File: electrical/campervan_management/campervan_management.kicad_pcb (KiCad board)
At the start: 2 copper layers, 45 parts, among them J1 Duoetto Remote, J2 Input Flow Sensor, J3 Output Flow Sensor, J4 Battery Box, J5 Starter Battery, J6 Fuse and Switch Box, K1 G5Q-1, K2 G5Q-1, K3 G5Q-1, Q1 BC337, Q2 BC337, Q3 BC337, Q4 BC337, SW1 SW_Push, U1 RS485-TTL, U2 LM7805

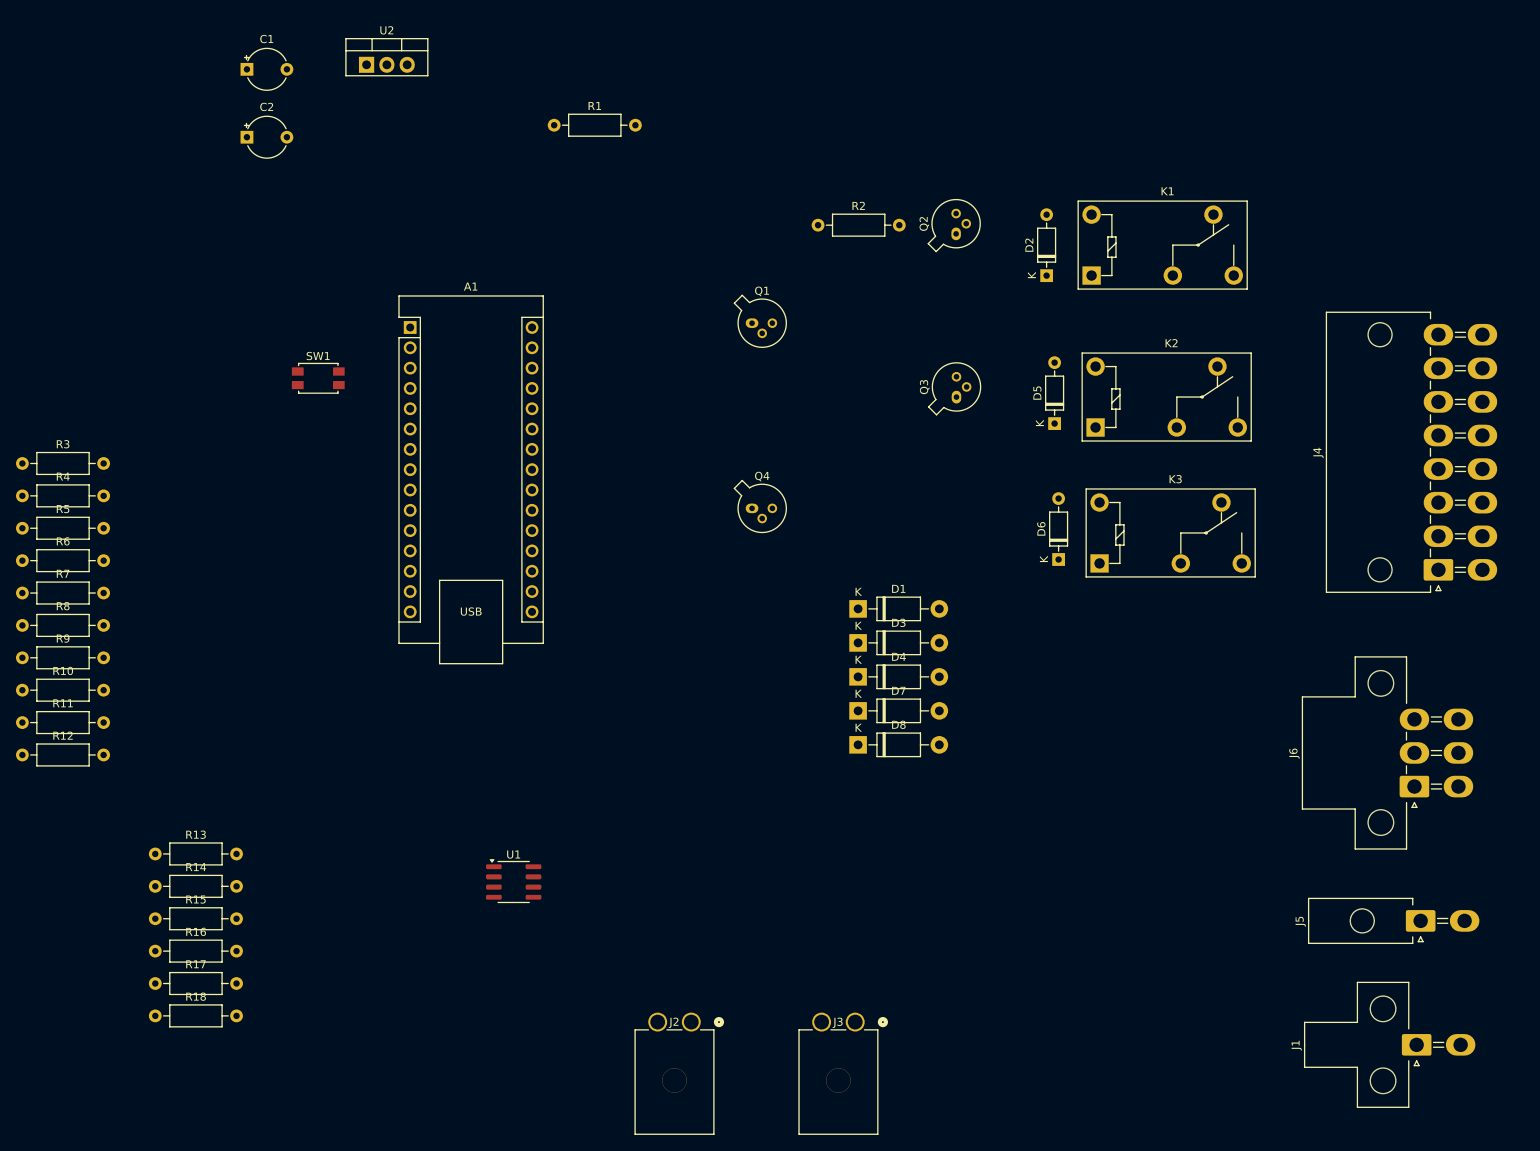
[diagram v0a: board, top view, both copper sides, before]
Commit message: First attempt at PCB design
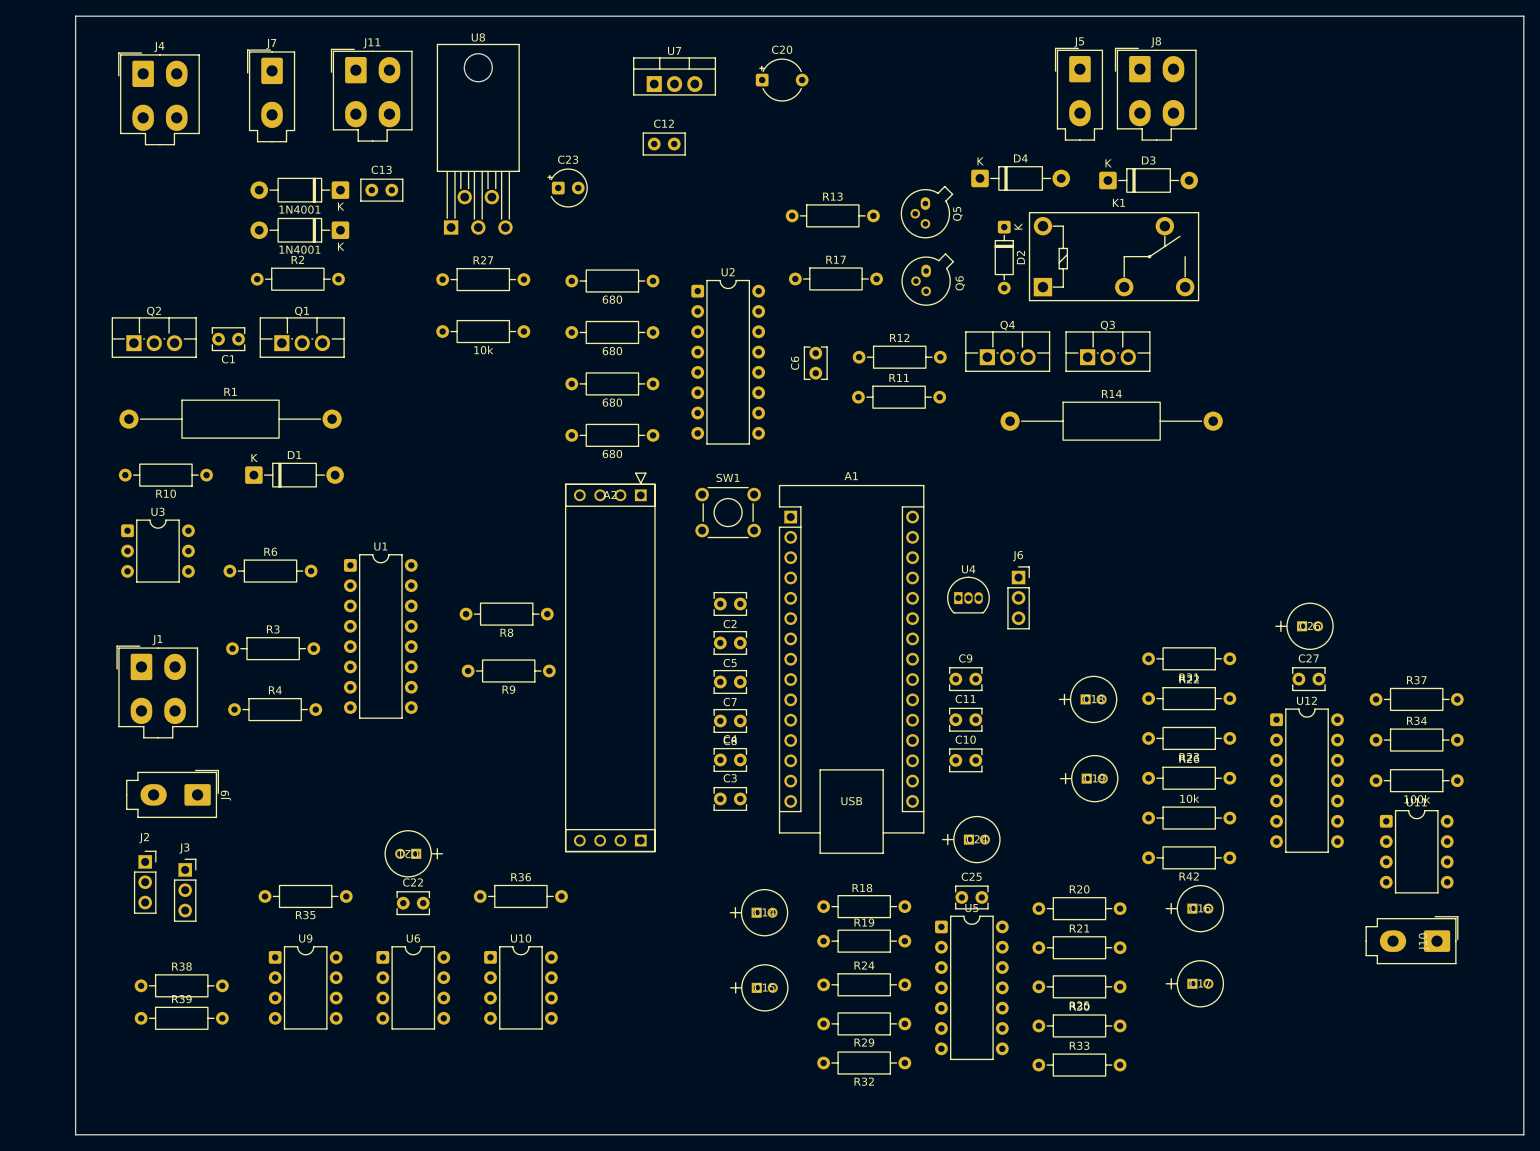
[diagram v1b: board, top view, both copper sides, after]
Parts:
- removed D7, D8: 1N4001, Diode_THT:D_DO-41_SOD81_P10.16mm_Horizontal
- removed K2, K3: G5Q-1, Relay_THT:Relay_SPDT_Omron-G5Q-1
- added A2: MAX485, CV_connector:RS485_MODULE, F.Cu at (111.3, 73.3)
- added C10: 100nF, Capacitor_THT:C_Disc_D3.8mm_W2.6mm_P2.50mm, F.Cu at (150.6, 106.4)
- added C11: 100nF, Capacitor_THT:C_Disc_D3.8mm_W2.6mm_P2.50mm, F.Cu at (150.6, 101.3)
- added C12: 0.33uF, Capacitor_THT:C_Disc_D5.0mm_W2.5mm_P2.50mm, F.Cu at (112.9, 29.4)
- added C13: 0.33uF, Capacitor_THT:C_Disc_D5.0mm_W2.5mm_P2.50mm, F.Cu at (77.6, 35.1)
- added C14: 1uF, CV_capacitor:CAP_NP_5X11_MTC, F.Cu at (125.7, 125.5)
- added C15: 1uF, CV_capacitor:CAP_NP_5X11_MTC, F.Cu at (125.8, 134.9)
- added C16: 1uF, CV_capacitor:CAP_NP_5X11_MTC, F.Cu at (180.2, 125.0)
- added C17: 1uF, CV_capacitor:CAP_NP_5X11_MTC, F.Cu at (180.2, 134.4)
- added C18: 1uF, CV_capacitor:CAP_NP_5X11_MTC, F.Cu at (166.9, 98.8)
- added C19: 1uF, CV_capacitor:CAP_NP_5X11_MTC, F.Cu at (167.0, 108.7)
- added C20: 0.1uF, Capacitor_THT:CP_Radial_Tantal_D5.0mm_P5.00mm, F.Cu at (126.4, 21.4)
- added C21: 1uF, CV_capacitor:CAP_NP_5X11_MTC, F.Cu at (83.2, 118.1)
- added C22: 100nF, Capacitor_THT:C_Disc_D3.8mm_W2.6mm_P2.50mm, F.Cu at (81.5, 124.3)
- added C23: 22uF, Capacitor_THT:CP_Radial_Tantal_D4.5mm_P2.50mm, F.Cu at (100.9, 34.9)
- added C24: 1uF, CV_capacitor:CAP_NP_5X11_MTC, F.Cu at (152.3, 116.3)
- added C25: 100nF, Capacitor_THT:C_Disc_D3.8mm_W2.6mm_P2.50mm, F.Cu at (151.4, 123.6)
- added C26: 1uF, CV_capacitor:CAP_NP_5X11_MTC, F.Cu at (193.9, 89.7)
- added C27: 100nF, Capacitor_THT:C_Disc_D3.8mm_W2.6mm_P2.50mm, F.Cu at (193.5, 96.3)
- added C3: 100nF, Capacitor_THT:C_Disc_D3.8mm_W2.6mm_P2.50mm, F.Cu at (121.2, 111.3)
- added C4: 100nF, Capacitor_THT:C_Disc_D3.8mm_W2.6mm_P2.50mm, F.Cu at (121.2, 106.4)
- added C5: 100nF, Capacitor_THT:C_Disc_D3.8mm_W2.6mm_P2.50mm, F.Cu at (123.7, 91.7)
- added C6: 100nF, Capacitor_THT:C_Disc_D3.8mm_W2.6mm_P2.50mm, F.Cu at (133.1, 58.0)
- added C7: 100nF, Capacitor_THT:C_Disc_D3.8mm_W2.6mm_P2.50mm, F.Cu at (123.7, 96.6)
- added C8: 100nF, Capacitor_THT:C_Disc_D3.8mm_W2.6mm_P2.50mm, F.Cu at (123.7, 101.5)
- added C9: 100nF, Capacitor_THT:C_Disc_D3.8mm_W2.6mm_P2.50mm, F.Cu at (150.6, 96.3)
- added J10: Starter Battery, Connector_Molex:Molex_Mini-Fit_Jr_5566-02A_2x01_P4.20mm_Vertical, F.Cu at (210.8, 129.0)
- added J11: Battery & Fuse, Connector_Molex:Molex_Mini-Fit_Jr_5566-04A_2x02_P4.20mm_Vertical, F.Cu at (75.6, 20.1)
- added J7: 12V Power, Connector_Molex:Molex_Mini-Fit_Jr_5566-02A_2x01_P4.20mm_Vertical, F.Cu at (65.1, 20.2)
- added J8: Relays, Connector_Molex:Molex_Mini-Fit_Jr_5566-04A_2x02_P4.20mm_Vertical, F.Cu at (173.7, 20.0)
- added J9: RS485, Connector_Molex:Molex_Mini-Fit_Jr_5566-02A_2x01_P4.20mm_Vertical, F.Cu at (55.8, 110.7)
- added Q5: 2N2222, Package_TO_SOT_THT:TO-18-3, F.Cu at (146.8, 36.8)
- added Q6: 2N2222, Package_TO_SOT_THT:TO-18-3, F.Cu at (146.9, 45.2)
- added R19: 10k, Resistor_THT:R_Axial_DIN0207_L6.3mm_D2.5mm_P10.16mm_Horizontal, F.Cu at (144.3, 129.0)
- added R20: 5k9, Resistor_THT:R_Axial_DIN0207_L6.3mm_D2.5mm_P10.16mm_Horizontal, F.Cu at (161.0, 125.0)
- added R21: 10k, Resistor_THT:R_Axial_DIN0207_L6.3mm_D2.5mm_P10.16mm_Horizontal, F.Cu at (161.0, 129.9)
- added R22: 5k9, Resistor_THT:R_Axial_DIN0207_L6.3mm_D2.5mm_P10.16mm_Horizontal, F.Cu at (174.8, 98.7)
- added R23: 10k, Resistor_THT:R_Axial_DIN0207_L6.3mm_D2.5mm_P10.16mm_Horizontal, F.Cu at (184.9, 103.7)
- added R24: 154k, Resistor_THT:R_Axial_DIN0207_L6.3mm_D2.5mm_P10.16mm_Horizontal, F.Cu at (134.1, 134.5)
- added R25: 154k, Resistor_THT:R_Axial_DIN0207_L6.3mm_D2.5mm_P10.16mm_Horizontal, F.Cu at (171.2, 134.7)
- added R26: 154k, Resistor_THT:R_Axial_DIN0207_L6.3mm_D2.5mm_P10.16mm_Horizontal, F.Cu at (174.8, 108.7)
- added R27: 68k, Resistor_THT:R_Axial_DIN0207_L6.3mm_D2.5mm_P10.16mm_Horizontal, F.Cu at (86.5, 46.3)
- added R28: 10k, Resistor_THT:R_Axial_DIN0207_L6.3mm_D2.5mm_P10.16mm_Horizontal, F.Cu at (96.6, 52.8)
- added R29: 154k, Resistor_THT:R_Axial_DIN0207_L6.3mm_D2.5mm_P10.16mm_Horizontal, F.Cu at (144.3, 139.4)
- added R30: 154k, Resistor_THT:R_Axial_DIN0207_L6.3mm_D2.5mm_P10.16mm_Horizontal, F.Cu at (161.0, 139.6)
- added R31: 154k, Resistor_THT:R_Axial_DIN0207_L6.3mm_D2.5mm_P10.16mm_Horizontal, F.Cu at (184.9, 93.7)
- added R32: 22k, Resistor_THT:R_Axial_DIN0207_L6.3mm_D2.5mm_P10.16mm_Horizontal, F.Cu at (144.3, 144.3)
- added R33: 22k, Resistor_THT:R_Axial_DIN0207_L6.3mm_D2.5mm_P10.16mm_Horizontal, F.Cu at (161.0, 144.5)
- added R34: 22k, Resistor_THT:R_Axial_DIN0207_L6.3mm_D2.5mm_P10.16mm_Horizontal, F.Cu at (203.2, 103.9)
- added R35: 1k2, Resistor_THT:R_Axial_DIN0207_L6.3mm_D2.5mm_P10.16mm_Horizontal, F.Cu at (74.4, 123.4)
- added R36: 1k2, Resistor_THT:R_Axial_DIN0207_L6.3mm_D2.5mm_P10.16mm_Horizontal, F.Cu at (91.2, 123.4)
- added R37: 1k2, Resistor_THT:R_Axial_DIN0207_L6.3mm_D2.5mm_P10.16mm_Horizontal, F.Cu at (203.2, 98.8)
- added R38: 100k, Resistor_THT:R_Axial_DIN0207_L6.3mm_D2.5mm_P10.16mm_Horizontal, F.Cu at (48.8, 134.6)
- added R39: 100k, Resistor_THT:R_Axial_DIN0207_L6.3mm_D2.5mm_P10.16mm_Horizontal, F.Cu at (48.8, 138.7)
- added R40: 100k, Resistor_THT:R_Axial_DIN0207_L6.3mm_D2.5mm_P10.16mm_Horizontal, F.Cu at (213.4, 109.0)
- added R41: 10k, Resistor_THT:R_Axial_DIN0207_L6.3mm_D2.5mm_P10.16mm_Horizontal, F.Cu at (174.8, 113.6)
- added R42: 10k, Resistor_THT:R_Axial_DIN0207_L6.3mm_D2.5mm_P10.16mm_Horizontal, F.Cu at (184.9, 118.6)
- added U10: IL300, Package_DIP:DIP-8_W7.62mm, F.Cu at (92.5, 131.1)
- added U11: IL300, Package_DIP:DIP-8_W7.62mm, F.Cu at (204.5, 114.0)
- added U12: MCP6004, Package_DIP:DIP-14_W7.62mm, F.Cu at (190.8, 101.3)
- added U3: CNY17-3, Package_DIP:DIP-6_W7.62mm, F.Cu at (47.1, 77.7)
- added U4: DS18B20, Package_TO_SOT_THT:TO-92_Inline, F.Cu at (151.0, 86.1)
- added U5: MCP6004, Package_DIP:DIP-14_W7.62mm, F.Cu at (148.8, 127.3)
- added U6: MCP6002-xP, Package_DIP:DIP-8_W7.62mm, F.Cu at (79.0, 131.1)
- added U7: LM7805, Package_TO_SOT_THT:TO-220-3_Vertical, F.Cu at (112.9, 21.9)
- added U8: BA00, Package_TO_SOT_THT:TO-220-5_P3.4x3.8mm_StaggerOdd_Lead7.13mm_TabDown, F.Cu at (87.5, 39.8)
- added U9: IL300, Package_DIP:DIP-8_W7.62mm, F.Cu at (65.5, 131.1)
- C1: value 0.33uF -> 100nF; footprint Capacitor_THT:CP_Radial_Tantal_D5.0mm_P5.00mm -> Capacitor_THT:C_Disc_D3.8mm_W2.6mm_P2.50mm
- C2: value 0.1uF -> 100nF; footprint Capacitor_THT:CP_Radial_Tantal_D5.0mm_P5.00mm -> Capacitor_THT:C_Disc_D3.8mm_W2.6mm_P2.50mm
- D5, D6: value 1N914 -> 1N4001; footprint Diode_THT:D_DO-35_SOD27_P7.62mm_Horizontal -> Diode_THT:D_DO-41_SOD81_P10.16mm_Horizontal
- J1: value Duoetto Remote -> Fans; footprint Connector_Molex:Molex_Mini-Fit_Jr_5569-02A1_2x01_P4.20mm_Horizontal -> Connector_Molex:Molex_Mini-Fit_Jr_5566-04A_2x02_P4.20mm_Vertical
- J2, J3: footprint Connector_Molex:CONN_SD-172648-0000_02_MOL -> Connector_PinSocket_2.54mm:PinSocket_1x03_P2.54mm_Vertical
- J4: value Battery Box -> Battery 2; footprint Connector_Molex:Molex_Mini-Fit_Jr_5569-16A2_2x08_P4.20mm_Horizontal -> Connector_Molex:Molex_Mini-Fit_Jr_5566-04A_2x02_P4.20mm_Vertical
- J5: value Starter Battery -> Power On/Off; footprint Connector_Molex:Molex_Mini-Fit_Jr_5569-02A2_2x01_P4.20mm_Horizontal -> Connector_Molex:Molex_Mini-Fit_Jr_5566-02A_2x01_P4.20mm_Vertical
- J6: value Fuse and Switch Box -> Temp; footprint Connector_Molex:Molex_Mini-Fit_Jr_5569-06A1_2x03_P4.20mm_Horizontal -> Connector_PinSocket_2.54mm:PinSocket_1x03_P2.54mm_Vertical
- K1: value G5Q-1 -> G5V-1
- Q1, Q2, Q3, Q4: value BC337 -> STP40NF30L; footprint Package_TO_SOT_THT:TO-18-3 -> Package_TO_SOT_THT:TO-220F-3_Vertical
- R1: value 150 -> 100 2W; footprint Resistor_THT:R_Axial_DIN0207_L6.3mm_D2.5mm_P10.16mm_Horizontal -> Resistor_THT:R_Axial_DIN0414_L11.9mm_D4.5mm_P25.40mm_Horizontal
- R10, R8: value 10K 1% -> 180
- R11: value 35.7K 1% -> 4k7
- R12: value 10K 1% -> 4k7
- R14: value 35.7K 1% -> 41R 2W; footprint Resistor_THT:R_Axial_DIN0207_L6.3mm_D2.5mm_P10.16mm_Horizontal -> Resistor_THT:R_Axial_DIN0414_L11.9mm_D4.5mm_P25.40mm_Horizontal
- R15: value 10K 1% -> 680
- R16: value 150 -> 680
- R17: value 35.7K 1% -> 150
- R18: value 10K 1% -> 5k9
- R2: value 1k -> 1M
- R3: value 35.7K 1% -> 47k
- R4: value 10K 1% -> 47k
- R5, R7: value 35.7K 1% -> 680
- R6: value 10K 1% -> 2k2
- R9: value 35.7K 1% -> 180
- SW1: footprint Button_Switch_SMD:SW_SPST_EVQP2 -> Button_Switch_THT:SW_TH_Tactile_Omron_B3F-102x
- U1: value RS485-TTL -> ILQ615-3; footprint Package_SO:SOIC-8_3.9x4.9mm_P1.27mm -> Package_DIP:DIP-16_W7.62mm
- U2: value LM7805 -> ILQ615-3; footprint Package_TO_SOT_THT:TO-220-3_Vertical -> Package_DIP:DIP-16_W7.62mm
- moved J4 173.4 mm to (49.0, 20.6), turned to 0 degrees
- moved J1 166.3 mm to (48.8, 94.7), turned to 0 degrees
- moved R14 121.7 mm to (157.4, 64.0)
- moved R17 119.0 mm to (130.6, 46.2)
- moved R12 115.9 mm to (138.6, 56.0)
- moved J5 114.7 mm to (166.2, 20.0), turned to 0 degrees
- moved R13 112.7 mm to (130.2, 38.3)
- moved R11 112.2 mm to (138.5, 61.0)
- moved Q2 103.7 mm to (47.9, 54.3), turned to 0 degrees
- moved D6 98.8 mm to (73.7, 40.1), turned to 180 degrees
- moved R18 94.7 mm to (144.3, 124.7), turned to 180 degrees
- moved D5 94.0 mm to (73.7, 35.1), turned to 180 degrees
- moved R15 91.4 mm to (112.8, 59.4), turned to 180 degrees
- moved R16 89.6 mm to (112.8, 65.8), turned to 180 degrees
- moved J3 85.9 mm to (54.3, 120.1)
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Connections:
- A1 pad 1: Net-(A1-D1/TX) -> /Tx
- A1 pad 10: Net-(A1-D7) -> /Solar Charge Battery 2 On
- A1 pad 11: /Battery 2 On/Off Switch Sensor -> Net-(A1-D8)
- A1 pad 12: /Battery 2 On/Off -> Net-(A1-D9)
- A1 pad 13: /12V Power On/Off -> Net-(A1-D10/CS)
- A1 pad 14: unconnected-(A1-D11/COPI-Pad14) -> Net-(A1-D11/COPI)
- A1 pad 15: unconnected-(A1-D12/CIPO-Pad15) -> /Input Flow Sensor
- A1 pad 16: Net-(A1-D13/SCK) -> /Output Flow Sensor
- A1 pad 2: Net-(A1-D0/RX) -> /Rx
- A1 pad 22: Net-(A1-A3) -> /Battery 2 On/Off
- A1 pad 23: /Battery Box Temp Sensor -> /Batteries On
- A1 pad 26: /Starter Battery Sensor -> Net-(A1-A7)
- A1 pad 29: GND -> GNDD
- A1 pad 30: VIN -> VCC_MM_9V5
- A1 pad 4: GND -> GNDD
- A1 pad 5: Net-(A1-D2) -> /En
- A1 pad 6: Net-(A1-D3) -> /Battery 2 On/Off Switch Sensor
- A1 pad 7: Net-(A1-D4) -> /Solar Charge Battery 2 Switch Sensor
- A1 pad 8: unconnected-(A1-D5-Pad8) -> /Battery 1 Fuse Digital
- A1 pad 9: Net-(A1-D6) -> /Battery 2 Fuse Digital
- C1 pad 1: VIN -> Net-(Q1-G)
- C1 pad 2: GND -> Net-(J4-Pin_3)
- C2 pad 1: +5V -> /Battery 2 On/Off Switch Sensor
- C2 pad 2: GND -> GNDD
- D1 pad 1: +12V -> VIN
- D1 pad 2: /Solar Switch -> /Solar Charge Battery 2
- D2 pad 1: +12V -> VCC_3V3
- D5 pad 1: +12V -> VIN
- D6 pad 1: +12V -> VIN
- J1 pad 1: /RS485 Rx -> Net-(J1-Pin_1)
- J1 pad 2: /RS485 Tx -> Net-(J1-Pin_2)
- J2 pad 1: +5V -> VCC_3V3
- J2 pad 2: Net-(A1-D6) -> /Input Flow Sensor
- J3 pad 1: +5V -> VCC_3V3
- J3 pad 2: Net-(A1-D7) -> /Output Flow Sensor
- J4 pad 1: /RS485 Rx -> Net-(J4-Pin_1)
- J4 pad 2: /RS485 Tx -> VIN
- J4 pad 3: /Battery Box Fan -> Net-(J4-Pin_3)
- J4 pad 4: /Battery Box Temp Sensor -> GND
- J5 pad 1: Net-(J5-Pin_1) -> GND
- J5 pad 2: (no net) -> Net-(J5-Pin_2)
- J6 pad 1: Net-(J6-Pin_1) -> VCC_3V3
- J6 pad 2: Net-(J6-Pin_2) -> Net-(A1-A7)
- J6 pad 3: Net-(D6-A) -> GND
- K1 pad 1: +12V -> Net-(D2-A)
- K1 pad 2: +12V -> Net-(Q3-D)
- K1 pad 3: /Battery Box Fan -> Net-(D3-A)
- K1 pad 4: unconnected-(K1-Pad4) -> Net-(D4-A)
- K1 pad 5: Net-(D2-A) -> VCC_3V3
- Q1 pad 1: GND -> Net-(Q1-G)
- Q1 pad 2: Net-(Q1-B) -> /Solar Charge Battery 2
- Q1 pad 3: /Solar Switch -> GND
- Q2 pad 1: GND -> Net-(J4-Pin_3)
- Q2 pad 2: Net-(Q2-B) -> Net-(Q2-D)
- Q2 pad 3: Net-(D2-A) -> GND
- Q3 pad 1: GND -> Net-(Q3-G)
- Q3 pad 2: Net-(Q3-B) -> Net-(Q3-D)
- Q3 pad 3: Net-(D5-A) -> Net-(J5-Pin_2)
- Q4 pad 1: GND -> /Batteries On
- Q4 pad 2: Net-(Q4-B) -> Net-(Q4-D)
- Q4 pad 3: Net-(D6-A) -> GND
- R1 pad 1: Net-(Q1-B) -> Net-(Q2-D)
- R1 pad 2: Net-(A1-D3) -> /Solar Charge Battery 2
- R10 pad 1: Net-(A1-A2) -> /Solar Charge Battery 2 On
- R10 pad 2: GND -> Net-(R10-Pad2)
- R11 pad 1: /Battery 2 Out Sensor -> Net-(Q3-G)
- R11 pad 2: Net-(A1-A3) -> GND
- R12 pad 1: Net-(A1-A3) -> /Batteries On
- R13 pad 1: Net-(Q3-B) -> /Battery 2 On/Off Switch Sensor
- R13 pad 2: /12V Power On/Off -> Net-(Q5-B)
- R14 pad 1: Net-(J5-Pin_1) -> Net-(Q4-D)
- R14 pad 2: /Starter Battery Sensor -> Net-(Q3-D)
- R15 pad 1: /Starter Battery Sensor -> Net-(R15-Pad1)
- R15 pad 2: GND -> /Battery 1 Fuse Sensor
- R16 pad 1: /Battery 2 On/Off -> Net-(R16-Pad1)
- R16 pad 2: Net-(Q4-B) -> /Battery 2 Fuse Sensor
- R17 pad 1: Net-(D6-A) -> /Battery 2 On/Off
- R17 pad 2: /Battery 2 On/Off Switch Sensor -> Net-(Q6-B)
- R18 pad 1: /Battery 2 On/Off Switch Sensor -> Net-(A1-A0)
- R18 pad 2: GND -> Net-(U5A--)
- R2 pad 1: Net-(A1-D13/SCK) -> Net-(Q1-G)
- R2 pad 2: Net-(Q2-B) -> GND
- R3 pad 1: /Solar Switch -> +12V
- R3 pad 2: Net-(A1-D2) -> Net-(J1-Pin_2)
- R4 pad 1: Net-(A1-D2) -> +12V
- R4 pad 2: GND -> Net-(J1-Pin_1)
- R5 pad 1: /Battery 1 In Sensor -> Net-(R5-Pad1)
- R5 pad 2: Net-(A1-A0) -> Net-(J4-Pin_1)
- R6 pad 1: Net-(A1-A0) -> Net-(J4-Pin_3)
- R7 pad 1: /Battery 2 In Sensor -> Net-(R7-Pad1)
- R7 pad 2: Net-(A1-A1) -> Net-(J4-Pin_3)
- R8 pad 1: Net-(A1-A1) -> Net-(A1-D8)
- R8 pad 2: GND -> Net-(R8-Pad2)
- R9 pad 1: /Battery 1 Out Sensor -> Net-(A1-D9)
- R9 pad 2: Net-(A1-A2) -> Net-(R9-Pad2)
- SW1 pad 2: GND -> GNDD
- U1 pad 1: Net-(A1-D0/RX) -> Net-(R8-Pad2)
- U1 pad 2: Net-(A1-D4) -> GNDD
- U1 pad 3: Net-(A1-D4) -> GNDD
- U1 pad 4: Net-(A1-D1/TX) -> Net-(R9-Pad2)
- U1 pad 5: GND -> Net-(J1-Pin_2)
- U1 pad 6: /RS485 Rx -> GND
- U1 pad 7: /RS485 Tx -> GND
- U1 pad 8: +5V -> Net-(J1-Pin_1)
- U2 pad 1: VIN -> Net-(R5-Pad1)
- U2 pad 3: +5V -> GND
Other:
- board outline added: 181.1 x 139.9 mm
